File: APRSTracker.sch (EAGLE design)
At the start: 26 parts, among them IC1 TP4056

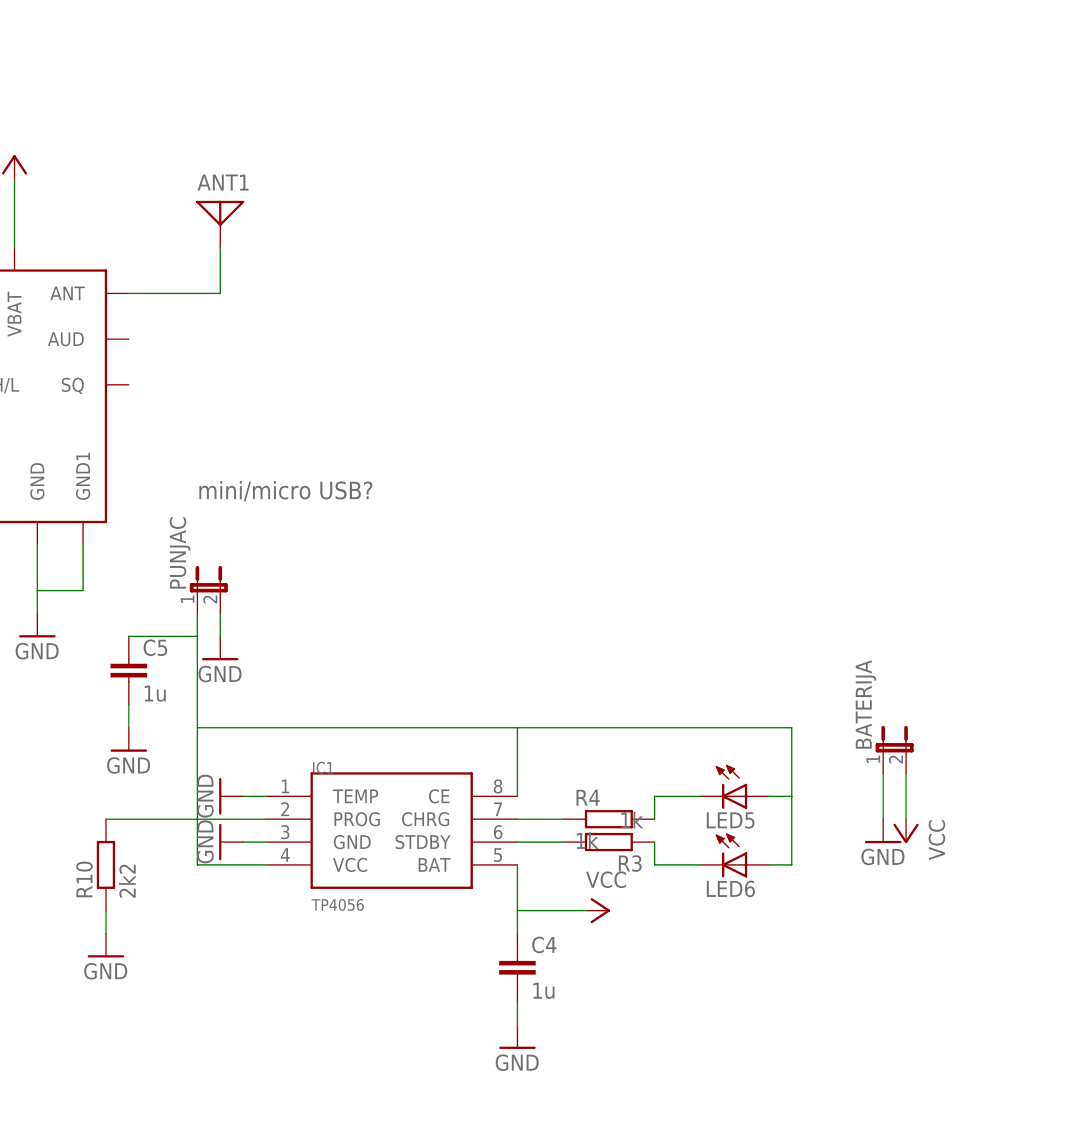
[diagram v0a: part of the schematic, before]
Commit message: sch update
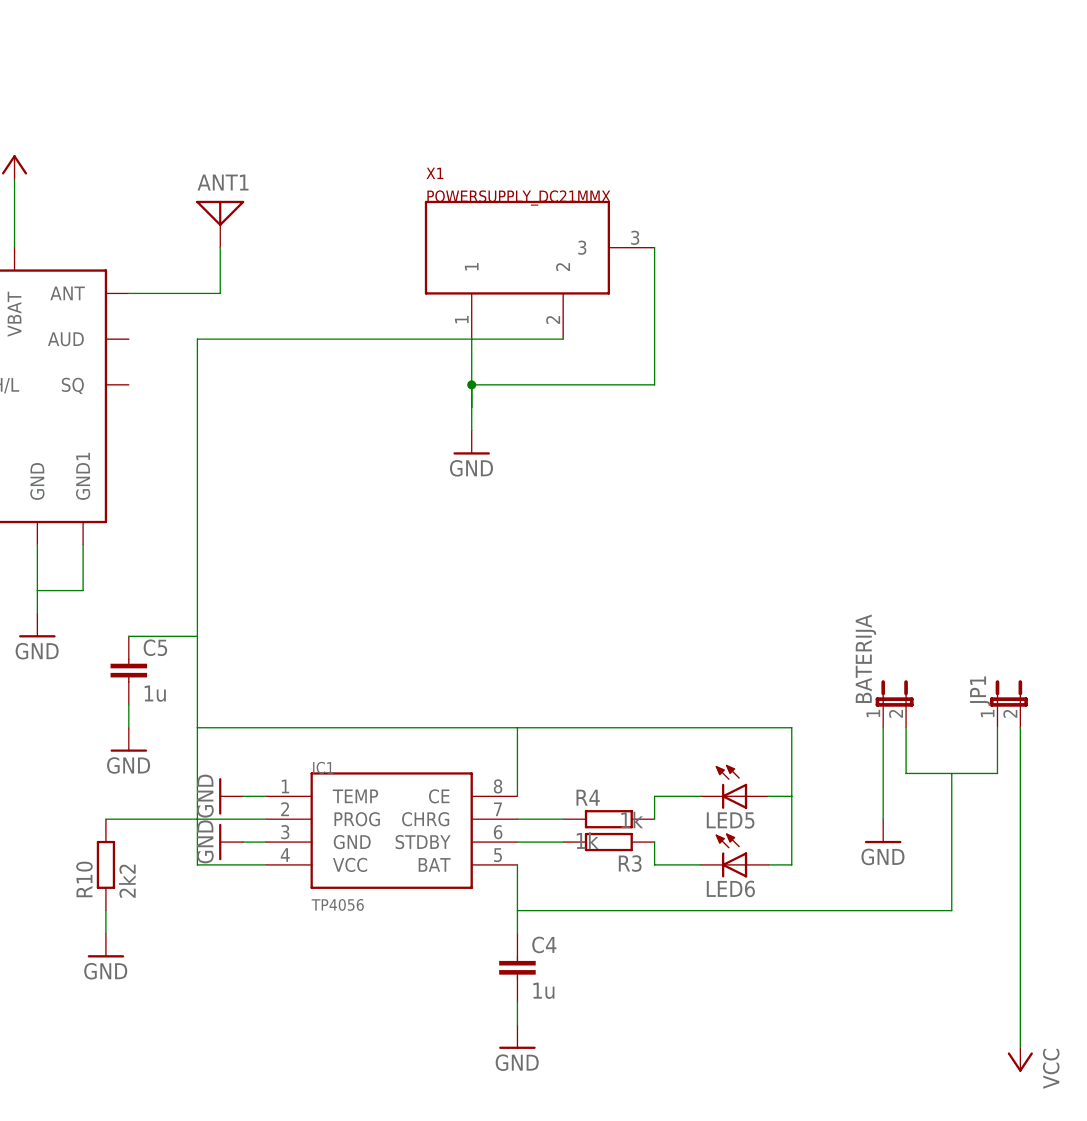
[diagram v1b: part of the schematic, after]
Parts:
- removed PUNJAC: (no value), jumper:JP1E
- added JP1: (no value), jumper:JP1E
- added X1: POWERSUPPLY_DC21MMX, SmartPrj:POWERSUPPLY_DC21MMX
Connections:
- new net N$31: BATERIJA.2, C4.1, IC1.BAT, JP1.1
- net GND: now also X1.1, X1.3; no longer PUNJAC.2
- net N$27: now also X1.2; no longer PUNJAC.1
- net VCC: now also JP1.2; no longer BATERIJA.2, C4.1, IC1.BAT
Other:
- note removed: "mini/micro USB?"
- moved on the sheet: BATERIJA
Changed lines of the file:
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@@
 <class number="0" name="default" width="0" drill="0">
+</class>
+<class number="1" name="power" width="0.6096" drill="0.6096">
+<clearance class="1" value="0.254"/>
 </class>
 <class number="2" name="gnd" width="0.3048" drill="0.5588">
@@
 <part name="C5" library="rcl" deviceset="C-EU" device="050-024X044" value="1u"/>
 <part name="BATERIJA" library="jumper" deviceset="JP1E" device=""/>
-<part name="P+6" library="supply1" deviceset="VCC" device=""/>
 <part name="GND6" library="supply1" deviceset="GND" device=""/>
-<part name="PUNJAC" library="jumper" deviceset="JP1E" device=""/>
 <part name="GND10" library="supply1" deviceset="GND" device=""/>
-<part name="GND11" library="supply1" deviceset="GND" device=""/>
 <part name="GND12" library="supply1" deviceset="GND" device=""/>
-<part name="P+7" library="supply1" deviceset="VCC" device=""/>
 <part name="GND13" library="supply1" deviceset="GND" device=""/>
 <part name="GND14" library="supply1" deviceset="GND" device=""/>
@@
 <part name="ANALOG" library="pinhead" deviceset="PINHD-1X5" device=""/>
 <part name="DIGITAL" library="pinhead" deviceset="PINHD-1X6" device=""/>
+<part name="GND19" library="supply1" deviceset="GND" device=""/>
+<part name="X1" library="SmartPrj" deviceset="POWERSUPPLY_DC21MM" device="X"/>
+<part name="JP1" library="jumper" deviceset="JP1E" device=""/>
+<part name="P+9" library="supply1" deviceset="VCC" device=""/>
 </parts>
 <sheets>
@@
 <text x="60.96" y="99.06" size="1.9304" layer="95">OSCILATOR</text>
 <text x="60.96" y="139.7" size="1.9304" layer="95">RESET</text>
-<text x="226.06" y="96.52" size="1.9304" layer="95">mini/micro USB?</text>
 </plain>
 <instances>
@@
 <instance part="C4" gate="G$1" x="261.62" y="45.72"/>
 <instance part="C5" gate="G$1" x="218.44" y="78.74"/>
-<instance part="BATERIJA" gate="A" x="302.26" y="68.58"/>
-<instance part="P+6" gate="VCC" x="304.8" y="58.42" rot="R180"/>
+<instance part="BATERIJA" gate="A" x="302.26" y="73.66"/>
 <instance part="GND6" gate="1" x="302.26" y="58.42"/>
-<instance part="PUNJAC" gate="A" x="226.06" y="86.36"/>
 <instance part="GND10" gate="1" x="215.9" y="45.72"/>
-<instance part="GND11" gate="1" x="228.6" y="78.74"/>
 <instance part="GND12" gate="1" x="228.6" y="58.42" rot="R270"/>
-<instance part="P+7" gate="VCC" x="271.78" y="50.8" rot="R270"/>
 <instance part="GND13" gate="1" x="261.62" y="35.56"/>
 <instance part="GND14" gate="1" x="218.44" y="68.58"/>
@@
 <instance part="ANALOG" gate="A" x="147.32" y="96.52"/>
 <instance part="DIGITAL" gate="A" x="147.32" y="76.2"/>
+<instance part="GND19" gate="1" x="256.54" y="101.6"/>
+<instance part="X1" gate="G$1" x="261.62" y="124.46" smashed="yes">
+<attribute name="NAME" x="251.46" y="132.08" size="1.27" layer="94"/>
+<attribute name="VALUE" x="251.46" y="129.54" size="1.27" layer="94"/>
+</instance>
+<instance part="JP1" gate="A" x="314.96" y="73.66"/>
+<instance part="P+9" gate="VCC" x="317.5" y="33.02" rot="R180"/>
 </instances>
 <busses>
@@
 <pinref part="BATERIJA" gate="A" pin="1"/>
 <pinref part="GND6" gate="1" pin="GND"/>
-<wire x1="302.26" y1="60.96" x2="302.26" y2="66.04" width="0.1524" layer="91"/>
+<wire x1="302.26" y1="60.96" x2="302.26" y2="71.12" width="0.1524" layer="91"/>
 </segment>
 <segment>
@@
 <pinref part="GND14" gate="1" pin="GND"/>
 <wire x1="218.44" y1="71.12" x2="218.44" y2="73.66" width="0.1524" layer="91"/>
-</segment>
-<segment>
-<pinref part="PUNJAC" gate="A" pin="2"/>
-<pinref part="GND11" gate="1" pin="GND"/>
-<wire x1="228.6" y1="81.28" x2="228.6" y2="83.82" width="0.1524" layer="91"/>
 </segment>
 <segment>
@@
 <pinref part="GND8" gate="1" pin="GND"/>
 <wire x1="187.96" y1="40.64" x2="187.96" y2="45.72" width="0.1524" layer="91"/>
+</segment>
+<segment>
+<wire x1="256.54" y1="114.3" x2="256.54" y2="109.22" width="0.1524" layer="91"/>
+<wire x1="256.54" y1="109.22" x2="256.54" y2="104.14" width="0.1524" layer="91"/>
+<wire x1="256.54" y1="109.22" x2="276.86" y2="109.22" width="0.1524" layer="91"/>
+<wire x1="276.86" y1="109.22" x2="276.86" y2="124.46" width="0.1524" layer="91"/>
+<wire x1="256.54" y1="106.68" x2="256.54" y2="109.22" width="0.1524" layer="91"/>
+<junction x="256.54" y="109.22"/>
+<pinref part="X1" gate="G$1" pin="1"/>
+<pinref part="GND19" gate="1" pin="GND"/>
+<pinref part="X1" gate="G$1" pin="3"/>
 </segment>
 </net>
@@
 <net name="VCC" class="0">
 <segment>
-<pinref part="BATERIJA" gate="A" pin="2"/>
-<pinref part="P+6" gate="VCC" pin="VCC"/>
-<wire x1="304.8" y1="60.96" x2="304.8" y2="66.04" width="0.1524" layer="91"/>
-</segment>
-<segment>
-<pinref part="IC1" gate="G$1" pin="BAT"/>
-<pinref part="C4" gate="G$1" pin="1"/>
-<wire x1="261.62" y1="55.88" x2="261.62" y2="50.8" width="0.1524" layer="91"/>
-<pinref part="P+7" gate="VCC" pin="VCC"/>
-<wire x1="261.62" y1="50.8" x2="261.62" y2="48.26" width="0.1524" layer="91"/>
-<wire x1="269.24" y1="50.8" x2="261.62" y2="50.8" width="0.1524" layer="91"/>
-</segment>
-<segment>
 <pinref part="R1" gate="G$1" pin="2"/>
 <wire x1="81.28" y1="139.7" x2="81.28" y2="132.08" width="0.1524" layer="91"/>
@@
 <wire x1="187.96" y1="78.74" x2="187.96" y2="73.66" width="0.1524" layer="91"/>
 </segment>
+<segment>
+<pinref part="JP1" gate="A" pin="2"/>
+<pinref part="P+9" gate="VCC" pin="VCC"/>
+<wire x1="317.5" y1="35.56" x2="317.5" y2="71.12" width="0.1524" layer="91"/>
+</segment>
 </net>
 <net name="N$18" class="0">
@@
 <wire x1="233.68" y1="55.88" x2="226.06" y2="55.88" width="0.1524" layer="91"/>
 <wire x1="226.06" y1="55.88" x2="226.06" y2="71.12" width="0.1524" layer="91"/>
-<pinref part="PUNJAC" gate="A" pin="1"/>
 <wire x1="226.06" y1="71.12" x2="226.06" y2="81.28" width="0.1524" layer="91"/>
 <pinref part="IC1" gate="G$1" pin="CE"/>
-<wire x1="226.06" y1="81.28" x2="226.06" y2="83.82" width="0.1524" layer="91"/>
 <wire x1="261.62" y1="63.5" x2="261.62" y2="71.12" width="0.1524" layer="91"/>
 <wire x1="261.62" y1="71.12" x2="226.06" y2="71.12" width="0.1524" layer="91"/>
@@
 <pinref part="C5" gate="G$1" pin="1"/>
 <wire x1="218.44" y1="81.28" x2="226.06" y2="81.28" width="0.1524" layer="91"/>
+<pinref part="X1" gate="G$1" pin="2"/>
+<wire x1="266.7" y1="114.3" x2="226.06" y2="114.3" width="0.1524" layer="91"/>
+<wire x1="226.06" y1="114.3" x2="226.06" y2="81.28" width="0.1524" layer="91"/>
 </segment>
 </net>
@@
 </segment>
 </net>
+<net name="N$31" class="0">
+<segment>
+<pinref part="IC1" gate="G$1" pin="BAT"/>
+<pinref part="C4" gate="G$1" pin="1"/>
+<wire x1="261.62" y1="55.88" x2="261.62" y2="50.8" width="0.1524" layer="91"/>
+<wire x1="261.62" y1="50.8" x2="261.62" y2="48.26" width="0.1524" layer="91"/>
+<pinref part="BATERIJA" gate="A" pin="2"/>
+<wire x1="304.8" y1="71.12" x2="304.8" y2="66.04" width="0.1524" layer="91"/>
+<wire x1="304.8" y1="66.04" x2="309.88" y2="66.04" width="0.1524" layer="91"/>
+<pinref part="JP1" gate="A" pin="1"/>
+<wire x1="309.88" y1="66.04" x2="314.96" y2="66.04" width="0.1524" layer="91"/>
+<wire x1="314.96" y1="66.04" x2="314.96" y2="71.12" width="0.1524" layer="91"/>
+<wire x1="261.62" y1="50.8" x2="309.88" y2="50.8" width="0.1524" layer="91"/>
+<wire x1="309.88" y1="50.8" x2="309.88" y2="66.04" width="0.1524" layer="91"/>
+</segment>
+</net>
